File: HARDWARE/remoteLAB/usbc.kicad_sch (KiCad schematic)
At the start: 0 parts

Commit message: added symbols for display connector and BT part, added usb device to ioc
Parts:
- added C1: 10n, symbol Device:C
- added FB1: 1u, symbol Device:FerriteBead
- added P1: USB_C_Plug_USB2.0, Connector_USB:USB_C_Receptacle_HCTL_HC-TYPE-C-16P-01A, symbol Connector:USB_C_Receptacle_USB2.0_14P
- added R10: 1k, symbol Device:R_Small
- added R8, R9: 5k1, symbol Device:R_Small
- added U1: ADUM4160, Package_SO:SOIC-16W_7.5x10.3mm_P1.27mm, symbol Interface_USB:ADUM4160
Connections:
- new net: R10.1, U1.13 (SPD), U1.14 (VDD2), U1.16 (VBUS2)
- new net: R10.2, U1.12 (PIN)
- new net: P1.A5 (CC1), R8.2
- new net: FB1.2, P1.A4 (VBUS), P1.A9 (VBUS), P1.B4 (VBUS), P1.B9 (VBUS)
- new net: P1.B5 (CC2), R9.2
- new net +5V: C1.1, FB1.1, U1.1 (VBUS1), U1.3 (VDD1), U1.4 (PDEN), U1.5 (SPU)
- new net GND: R8.1, R9.1, U1.15 (GND2), U1.9 (GND2)
- new net GND1: C1.2, P1.A1 (GND), P1.A12 (GND), P1.B1 (GND), P1.B12 (GND), P1.SH (SHIELD), U1.2 (GND1), U1.8 (GND1)
- new net USBC_D+: P1.A6 (D+), P1.B6 (D+), U1.7 (UD+)
- new net USBC_D-: P1.A7 (D-), P1.B7 (D-), U1.6 (UD-)
- new net uC_D+: U1.10 (DD+)
- new net uC_D-: U1.11 (DD-)

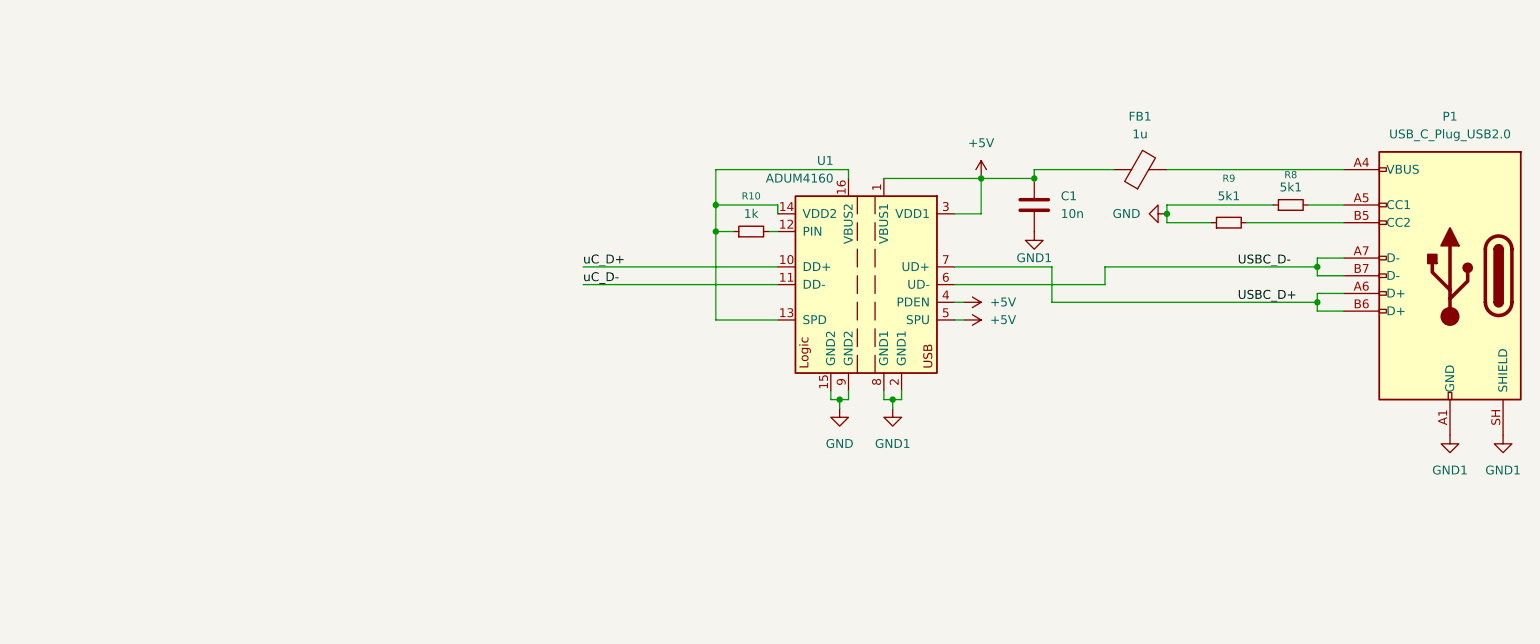
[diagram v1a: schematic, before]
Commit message: usb power isolation and input
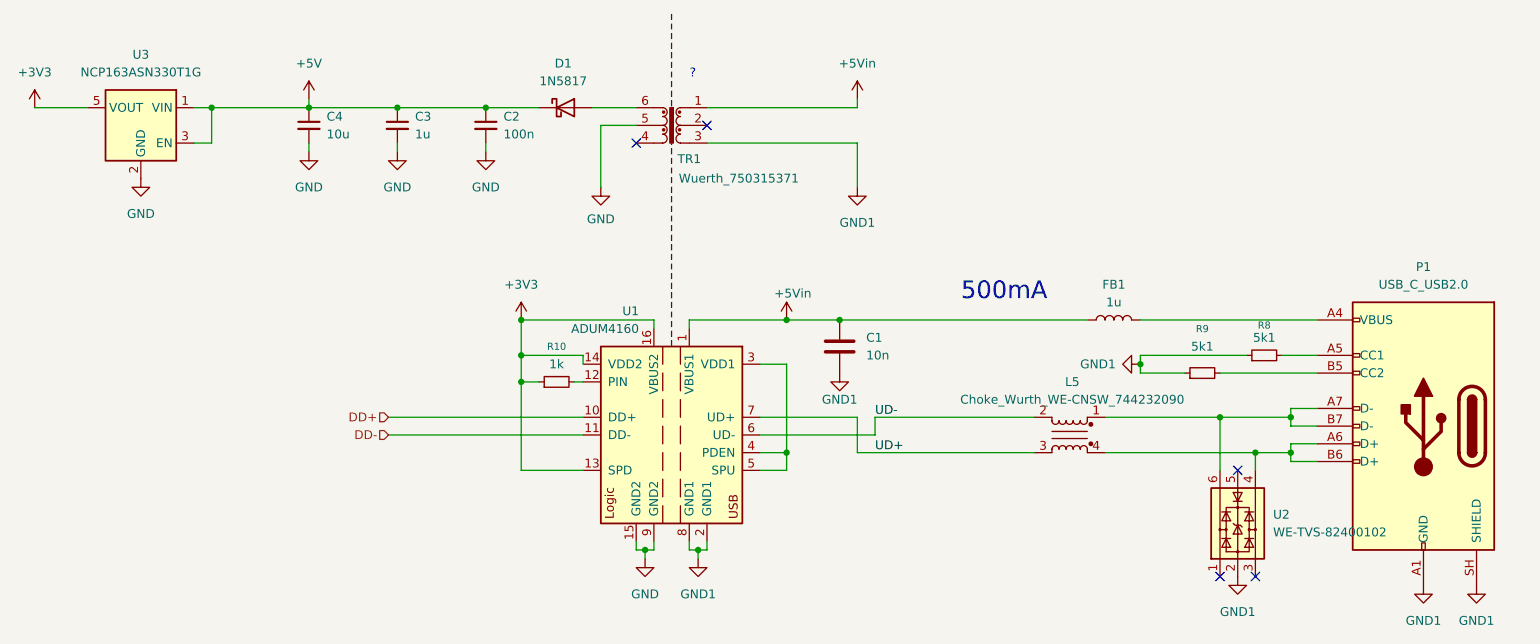
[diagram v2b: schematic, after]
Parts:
- added C2: 100n, symbol Device:C_Small
- added C3: 1u, symbol Device:C_Small
- added C4: 10u, symbol Device:C_Small
- added D1: 1N5817, Diode_THT:D_DO-41_SOD81_P10.16mm_Horizontal, symbol Diode:1N5817
- added L5: Choke_Wurth_WE-CNSW_744232090, Inductor_SMD:L_CommonMode_Wurth_WE-CNSW-1206, symbol Filter:Choke_Wurth_WE-CNSW_744232090
- added TR1: Wuerth_750315371, Transformer_SMD:Transformer_Wuerth_750315371, symbol Transformer:Wuerth_750315371
- added U2: WE-TVS-82400102, Package_TO_SOT_SMD:SOT-23-6_Handsoldering, symbol Power_Protection:WE-TVS-82400102
- added U3: NCP163ASN330T1G, Package_TO_SOT_SMD:SOT-23-5_HandSoldering, symbol Regulator_Linear:NCP163ASN330T1G
- FB1: symbol Device:FerriteBead -> Device:L
- P1: value USB_C_Plug_USB2.0 -> USB_C_USB2.0
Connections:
- net +5V: now also C2.1, C3.1, C4.1, D1.1 (K), U3.1 (VIN), U3.3 (EN); no longer C1.1, FB1.1, U1.1 (VBUS1), U1.3 (VDD1), U1.4 (PDEN), U1.5 (SPU)
- net GND: now also C2.2, C3.2, C4.2, TR1.5, U3.2 (GND); no longer R8.1, R9.1
- net GND1: now also R8.1, R9.1, TR1.3, U2.2
- net +3V3: now reaches R10.1, U1.13 (SPD), U1.14 (VDD2), U1.16 (VBUS2)
- net +3V3: now also U3.5 (VOUT)
- net USBC_D+: no longer names the net of P1.A6 (D+), P1.B6 (D+)
- net USBC_D+: now also L5.4, U2.4; no longer U1.7 (UD+)
- net USBC_D-: no longer names the net of P1.A7 (D-), P1.B7 (D-)
- net USBC_D-: now also L5.1, U2.6; no longer U1.6 (UD-)
- net uC_D+ renamed DD+
- net uC_D- renamed DD-
- new net: D1.2 (A), TR1.6
- new net: U1.3 (VDD1), U1.4 (PDEN), U1.5 (SPU)
- new net +5Vin: C1.1, FB1.1, TR1.1, U1.1 (VBUS1)
- new net UD+: L5.3, U1.7 (UD+)
- new net UD-: L5.2, U1.6 (UD-)
- no-connect marks 0 -> 5
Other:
- note added: "500mA"
- note added: "?"
- moved on the sheet: C1, P1, R10, R8, R9, U1
